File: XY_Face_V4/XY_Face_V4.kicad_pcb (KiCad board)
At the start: 4 copper layers, 83 x 98 mm, 32 parts, among them CN1 DF11-2DSA-4DP, J11 DF11-4DP-2DSA, J13 DF11-4DP-2DSA, J2 Conn_01x01, J3 Conn_01x01, J4 Conn_01x01, J5 Conn_01x01, Q2 CSD17576Q5B, U1 VEML7700, U2 TMP112xxDRL, U3 DRV2605LDGS, U4 TCA4311ADGKR, U5 5040500691, U6 5040500691

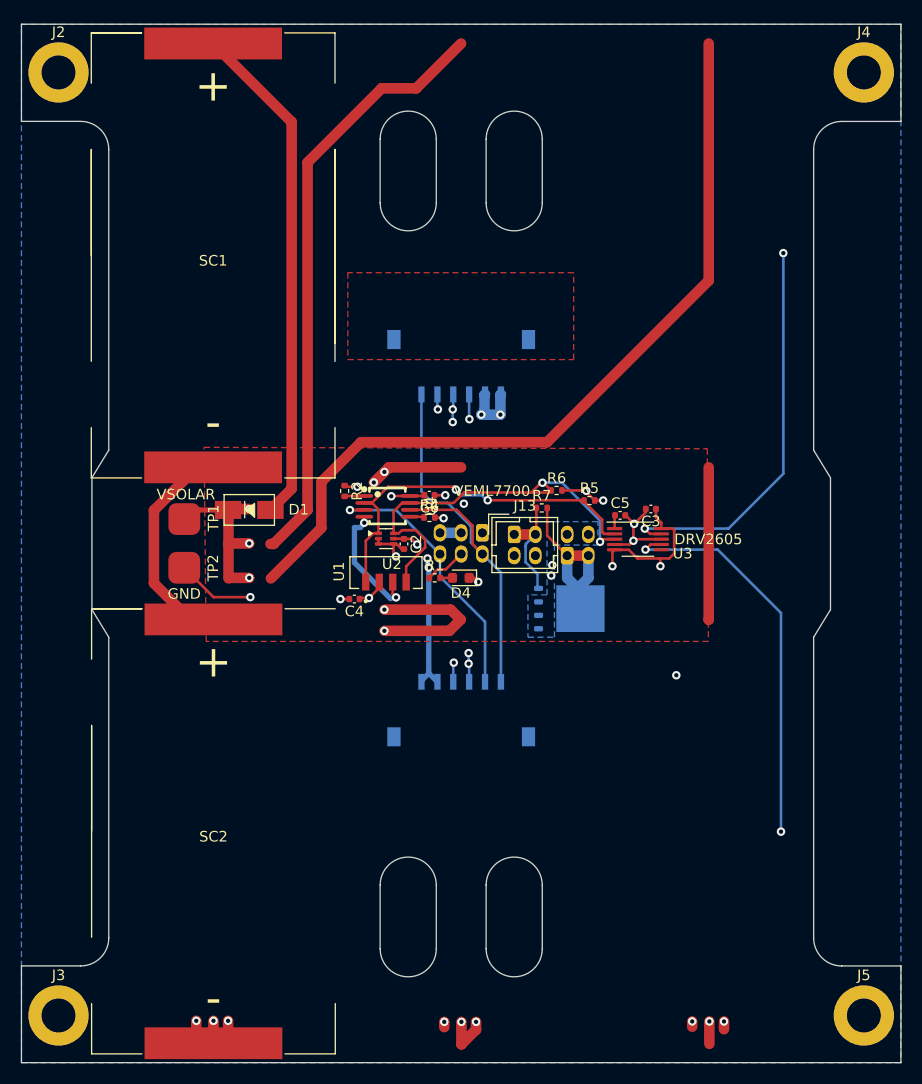
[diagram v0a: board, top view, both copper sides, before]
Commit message: V4: Added new Cells to Footprint
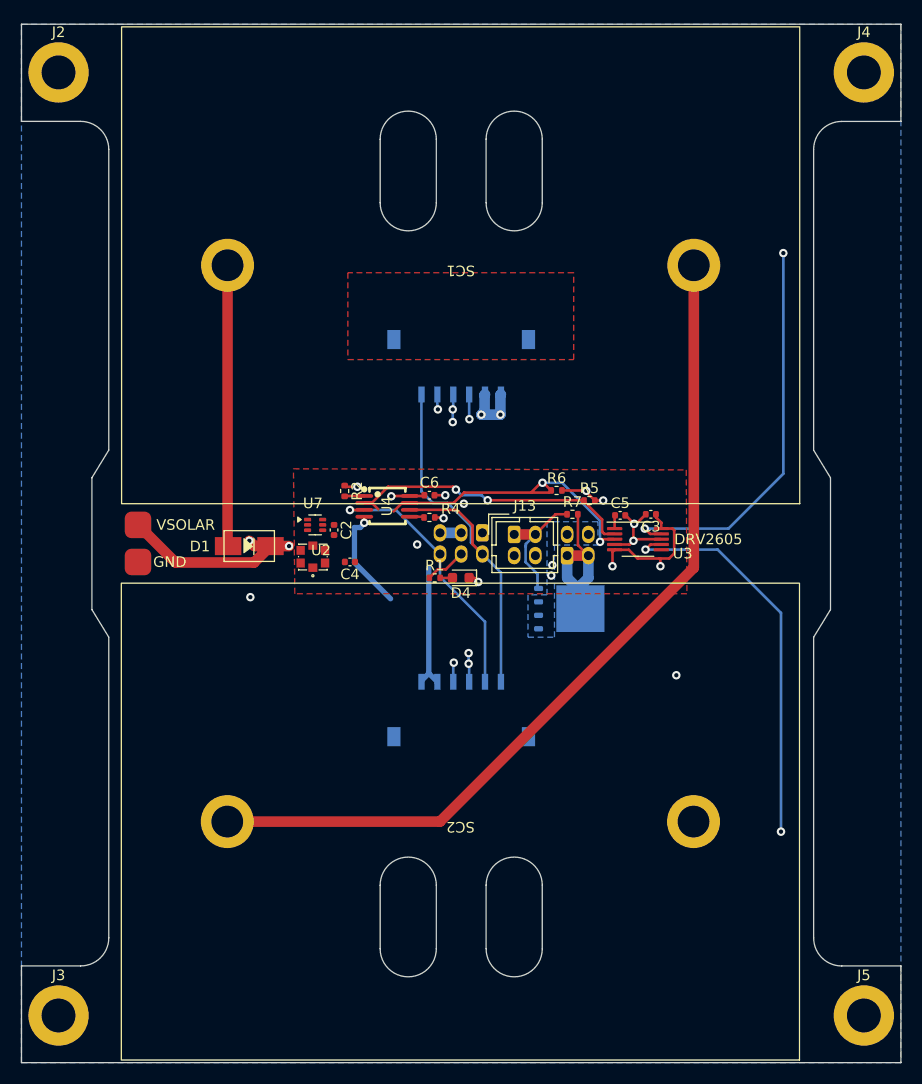
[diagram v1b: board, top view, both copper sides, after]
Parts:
- removed U1: VEML7700, VEML7700-TT:XDCR_VEML7700-TT
- added U7: VEML6031X00, easyeda2kicad:SENSOR-SMD_VEML6031X00, F.Cu at (130.5, 116.0)
- SC1, SC2: value SM101K07TF -> SM261K10TF; footprint SolarPanelBoards:KXOB101K08F-TR -> Solar_Cell_Library:SM261K10TF
- moved SC1 23.4 mm to (144.4, 88.5), turned to 180 degrees
- moved SC2 23.3 mm to (144.4, 141.0), turned to 180 degrees
- moved U2 6.81 mm to (130.7, 113.0)
- moved C2 6.73 mm to (132.5, 113.5)
- moved TP1 4.40 mm to (114.0, 113.0)
- moved TP2 4.39 mm to (114.0, 116.5)
- moved C4 3.53 mm to (134.0, 116.5)
- moved D1 3.41 mm to (124.5, 115.0), turned to 180 degrees
- moved R7 2.96 mm to (155.0, 112.0)
- moved C3 0.50 mm to (162.4, 112.0)
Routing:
- net Net-(D3-A): track 77.9 -> 0.00 mm
- net Net-(SC1--): track 21.2 -> 82.5 mm
- net Net-(D2-A): track 56.8 -> 0.00 mm
- net Net-(SC3--): track 39.9 -> 0.00 mm, vias 4 -> 0
- net GND: track 53.5 -> 26.9 mm, vias 21 -> 9
- net Net-(D1-A): track 47.9 -> 26.5 mm
- net Net-(SC5--): track 14.4 -> 0.00 mm
- net /SDA: track 39.0 -> 28.7 mm
- net VSOLAR: track 87.5 -> 77.6 mm, vias 7 -> 4
- net /SCL: track 36.0 -> 28.4 mm
- net Net-(J13-Pin_1): track 10.5 -> 11.8 mm
- net /RBF_High: track 18.1 -> 17.1 mm
- net +3V3: track 105.9 -> 105.3 mm, vias 13 -> 12
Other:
- board text removed: "VEML7700"
